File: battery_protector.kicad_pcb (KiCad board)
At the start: 4 copper layers, 140.5 x 121.1 mm, 104 parts, among them J1 TB005-762-02BE, J2 TB005-762-02BE, J3 USB_C_Receptacle_USB2.0_16P, J5 Conn_01x12, Q1 SQJQ184ER, Q2 SQJQ184ER, Q3 SQJQ184ER, Q4 SQJQ184ER, Q5 MMBT3904, Q6 MMBT3904, SW1 SW_DPDT_x2, SW2 PTS647SN50SMTR2_LFS, SW3 PTS647SN50SMTR2_LFS, U1 LMR38020SDDAR, U2 AP2112K-3.3, U3 TPS2116DRL, U4 CP2102N-Axx-xQFN28, U5 ESP32-C3-WROOM-02, U6 LIS3DH, U7 2ED4820EMXUMA2

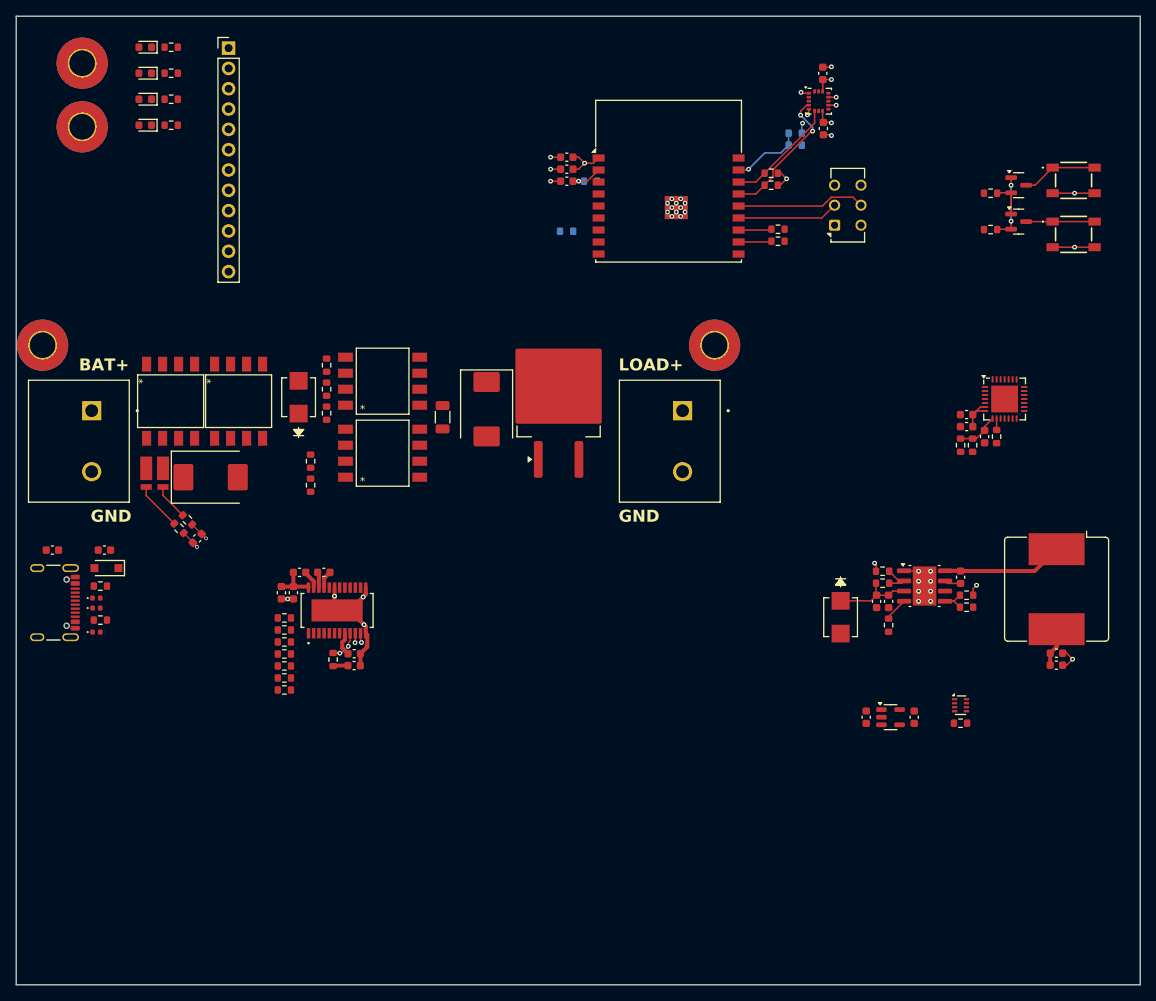
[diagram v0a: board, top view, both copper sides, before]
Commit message: route dc-dc
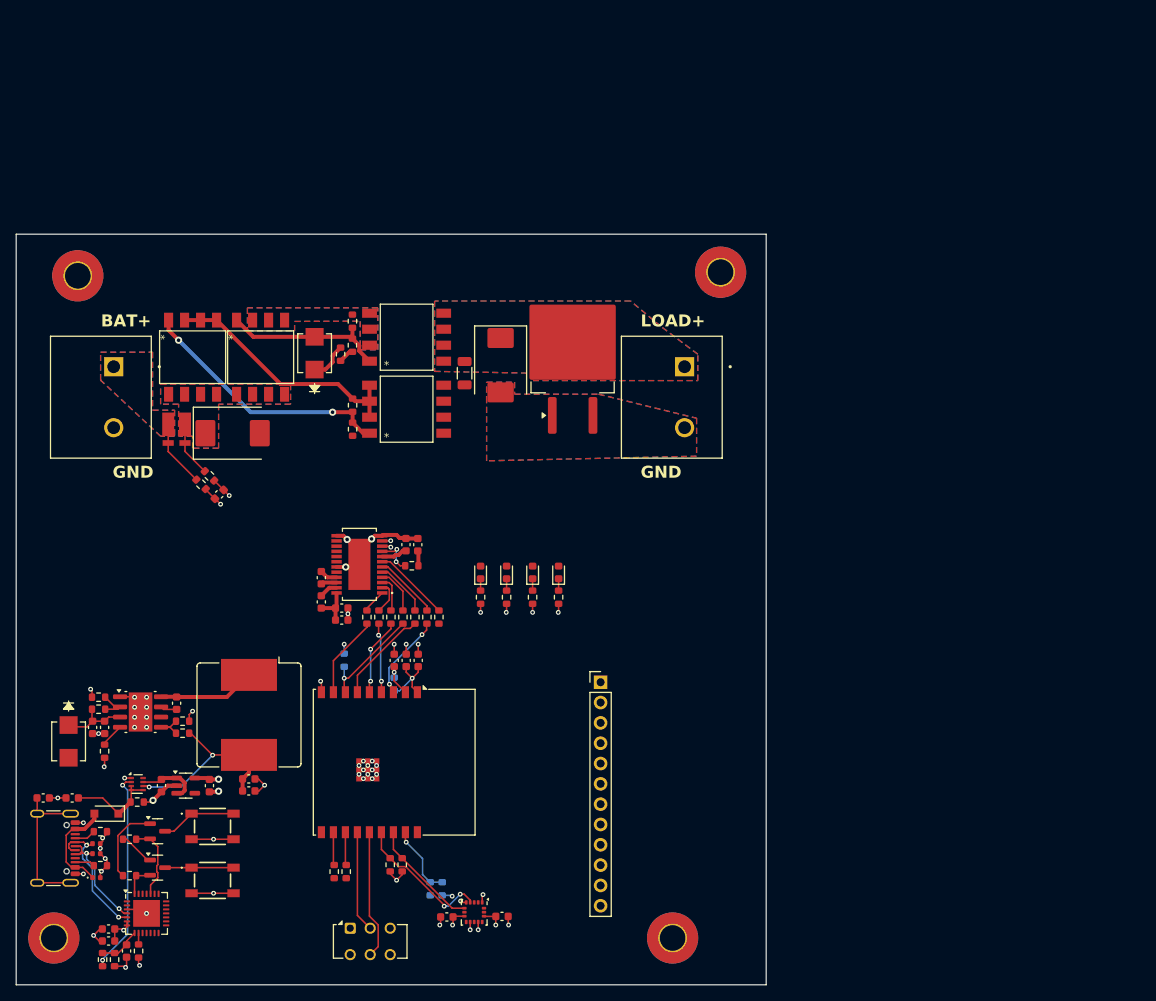
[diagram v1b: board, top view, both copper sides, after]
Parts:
- moved Q6 134.6 mm to (91.4, 136.3)
- moved R30 134.6 mm to (87.9, 137.3), turned to 0 degrees
- moved Q5 134.6 mm to (91.4, 131.8)
- moved R31 134.6 mm to (87.9, 132.8), turned to 0 degrees
- moved SW2 134.6 mm to (98.2, 131.2)
- moved SW3 134.6 mm to (98.2, 137.9)
- moved R23 125.1 mm to (84.5, 147.8)
- moved R24 125.1 mm to (86.0, 147.8)
- moved U4 125.1 mm to (90.0, 142.0)
- moved C11 125.1 mm to (87.5, 146.7)
- moved C22 125.1 mm to (85.2, 145.5)
- moved C23 125.1 mm to (85.2, 144.0)
- moved R26 125.1 mm to (89.0, 146.7)
- moved C16 112.7 mm to (134.4, 142.4), turned to 0 degrees
- moved U6 110.1 mm to (130.9, 141.9), turned to -90 degrees
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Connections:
- Q6 pad 3: /MCU/GD_SAFE -> /MCU/~{GD_SAFE}
- SW3 pad 1: /MCU/GD_SAFE -> /MCU/~{GD_SAFE}
- SW3 pad 2: /MCU/GD_SAFE -> /MCU/~{GD_SAFE}
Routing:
- net +5V0: track 0.00 -> 33.2 mm, vias 0 -> 2
- net Net-(Q1-G): track 0.00 -> 32.5 mm, vias 0 -> 2
- net /GateDriver/SOURCE_B: track 0.00 -> 31.3 mm
- net GND: track 51.7 -> 82.0 mm, vias 38 -> 58
- net Net-(D6-A): track 0.00 -> 20.5 mm
- net +5V0_board: track 4.83 -> 23.9 mm, vias 0 -> 2
- net Net-(J3-SHIELD): track 0.00 -> 19.0 mm
- net /MCU/~{GD_SAFE}: track 0.00 -> 18.9 mm
- net /DC-DC/USB_DN: track 0.00 -> 16.8 mm, vias 0 -> 2
- net /DC-DC/USB_DP: track 0.00 -> 14.5 mm, vias 0 -> 2
- net /~{CS}: track 0.00 -> 13.4 mm, vias 0 -> 1
- net Net-(D11-A1): track 0.00 -> 12.5 mm
- net /MOSI: track 0.00 -> 12.0 mm
- net +5V0_USB: track 0.00 -> 11.5 mm
- net /MISO: track 0.00 -> 10.8 mm, vias 0 -> 2
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- added copper zone on B.Cu, net /GateDriver/SOURCE_A
- added copper zone on F.Cu, net /GateDriver/SOURCE_A
- added copper zone on B.Cu, net BAT+
- added copper zone on F.Cu, net BAT+
- added copper zone on B.Cu, net GND
- added copper zone on F.Cu, net GND
- added copper zone on B.Cu, net LOAD+
- added copper zone on F.Cu, net LOAD+
- added copper zone on B.Cu, net Net-(D5-A1)
- added copper zone on F.Cu, net Net-(D5-A1)
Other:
- board size 140.5 x 121.1 mm -> 93.7 x 93.8 mm
- board text added: "Automatic ORing 5V->3.3V LDO"
- board text added: "BAT+->5V Buck"
- board text added: "ESP32 MCU"
- board text added: "Gate Driver"
- board text added: "USB-C"
- board text added: "USB-UART Bridge"
